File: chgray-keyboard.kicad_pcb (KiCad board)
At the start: 2 copper layers, 377.4 x 105.5 mm, 337 parts, among them SW1 30, SW10 22, SW11 32, SW12 52, SW13 02, SW14 12, SW15 03, SW16 13, SW17 23, SW18 33, SW19 43, SW2 40, SW20 53, SW21 24, SW22 34, SW23 54, SW24 04, SW25 14, SW26 05, SW27 15, SW28 25, SW29 35, SW3 50, SW30 45, SW31 26, SW32 36, SW33 46, SW34 56, SW35 06, SW36 16, SW37 07, SW38 17, SW39 27, SW4 00, SW40 37, SW41 57, SW42 28, SW43 38, SW44 48, SW45 58, SW46 08, SW47 18, SW48 09, SW49 19, SW5 01, SW50 29, SW51 39, SW52 49, SW53 010, SW54 110, SW55 210, SW56 310, SW57 410, SW58 510, SW59 111, SW6 11, SW60 211, SW61 311, SW62 411, SW63 511, SW64 111, SW65 211, SW66 311, SW67 411, SW68 511, SW69 111, SW7 21, SW70 211, SW71 311, SW72 411, SW73 511, SW8 41, SW9 51, U1 Teensy2.0_(C)

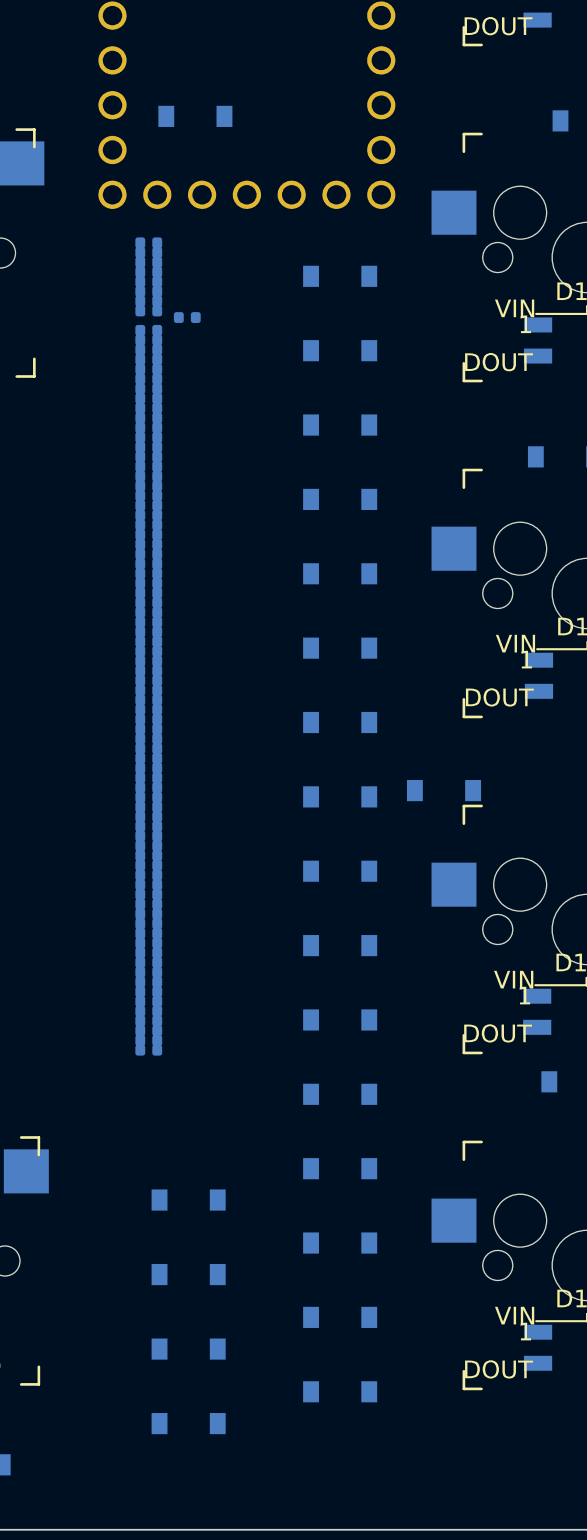
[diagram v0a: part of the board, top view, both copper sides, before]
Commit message: placed LED's ..mostly
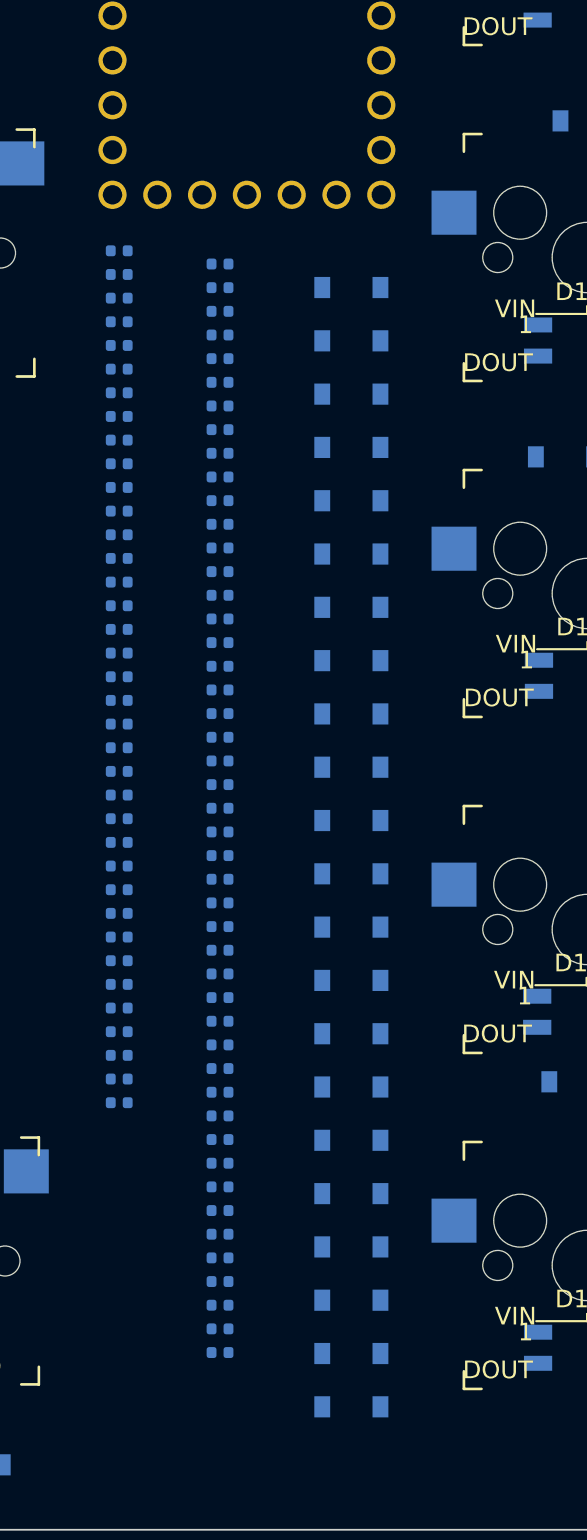
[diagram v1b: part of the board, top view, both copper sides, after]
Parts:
- moved D52 32.1 mm to (311.6, 137.5)
- moved C72 28.9 mm to (298.4, 162.6)
- moved C71 28.2 mm to (298.4, 161.3)
- moved C8 27.4 mm to (298.4, 159.9)
- moved C74 26.6 mm to (298.4, 158.6)
- moved C58 25.8 mm to (298.4, 157.2)
- moved C47 25.0 mm to (298.4, 155.9)
- moved C11 24.2 mm to (298.4, 154.6)
- moved C56 23.4 mm to (298.4, 153.2)
- moved C69 22.6 mm to (298.4, 151.9)
- moved C64 21.9 mm to (298.4, 150.5)
- moved D67 21.2 mm to (311.6, 161.7)
- moved C59 21.1 mm to (298.4, 149.2)
- moved C48 20.3 mm to (298.4, 147.8)
- moved C6 19.6 mm to (304.2, 115.0)
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
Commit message: routed
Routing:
- net LED_VDD: track 0.00 -> 2036.1 mm, vias 0 -> 16
- net /Keyboard Keys/KEY_ROW4: track 0.00 -> 613.3 mm, vias 0 -> 10
- net /Keyboard Keys/KEY_COL0: track 0.00 -> 556.2 mm, vias 0 -> 6
- net /Keyboard Keys/KEY_ROW3: track 0.00 -> 549.4 mm, vias 0 -> 10
- net /Keyboard Keys/KEY_ROW0: track 0.00 -> 521.1 mm, vias 0 -> 4
- net /Keyboard Keys/KEY_ROW5: track 0.00 -> 469.0 mm, vias 0 -> 9
- net /Keyboard Keys/KEY_ROW2: track 0.00 -> 455.8 mm, vias 0 -> 7
- net /Keyboard Keys/KEY_ROW1: track 0.00 -> 448.7 mm, vias 0 -> 8
- net /Keyboard Keys/KEY_COL13: track 0.00 -> 424.0 mm, vias 0 -> 8
- net /Keyboard Keys/KEY_COL2: track 0.00 -> 409.9 mm, vias 0 -> 7
- net Net-(C2-Pad1): track 0.00 -> 405.8 mm
- net /Keyboard Keys/KEY_COL1: track 0.00 -> 370.7 mm, vias 0 -> 6
- net Net-(C61-Pad1): track 0.00 -> 365.2 mm, vias 0 -> 4
- net Net-(D83-Pad1): track 0.00 -> 360.3 mm, vias 0 -> 2
- net Net-(D2-Pad1): track 0.00 -> 360.2 mm, vias 0 -> 2
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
